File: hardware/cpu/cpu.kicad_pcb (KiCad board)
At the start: 4 copper layers, 172.7 x 106.7 mm, 64 parts, among them J1 Conn_02x20_Odd_Even, J2 Conn_01x06, J3 Conn_01x06, J4 Conn_02x05_Odd_Even, J5 Conn_01x02, J6 Conn_02x20_Odd_Even, SW1 SW_Push, U1 74AS74, U10 74LS157, U11 Z80-DART, U12 74HCT04, U13 74LS32, U14 CTC, U15 74HCT04, U16 uA7805, U17 74AS74, U18 74AS74, U2 74LS138, U3 Z80CPU, U4 AT28C256, U5 74LS670, U6 74HC14, U7 74LS670, U8 AS6C4008, U9 Z80-PIO, X1 7.3728MHz

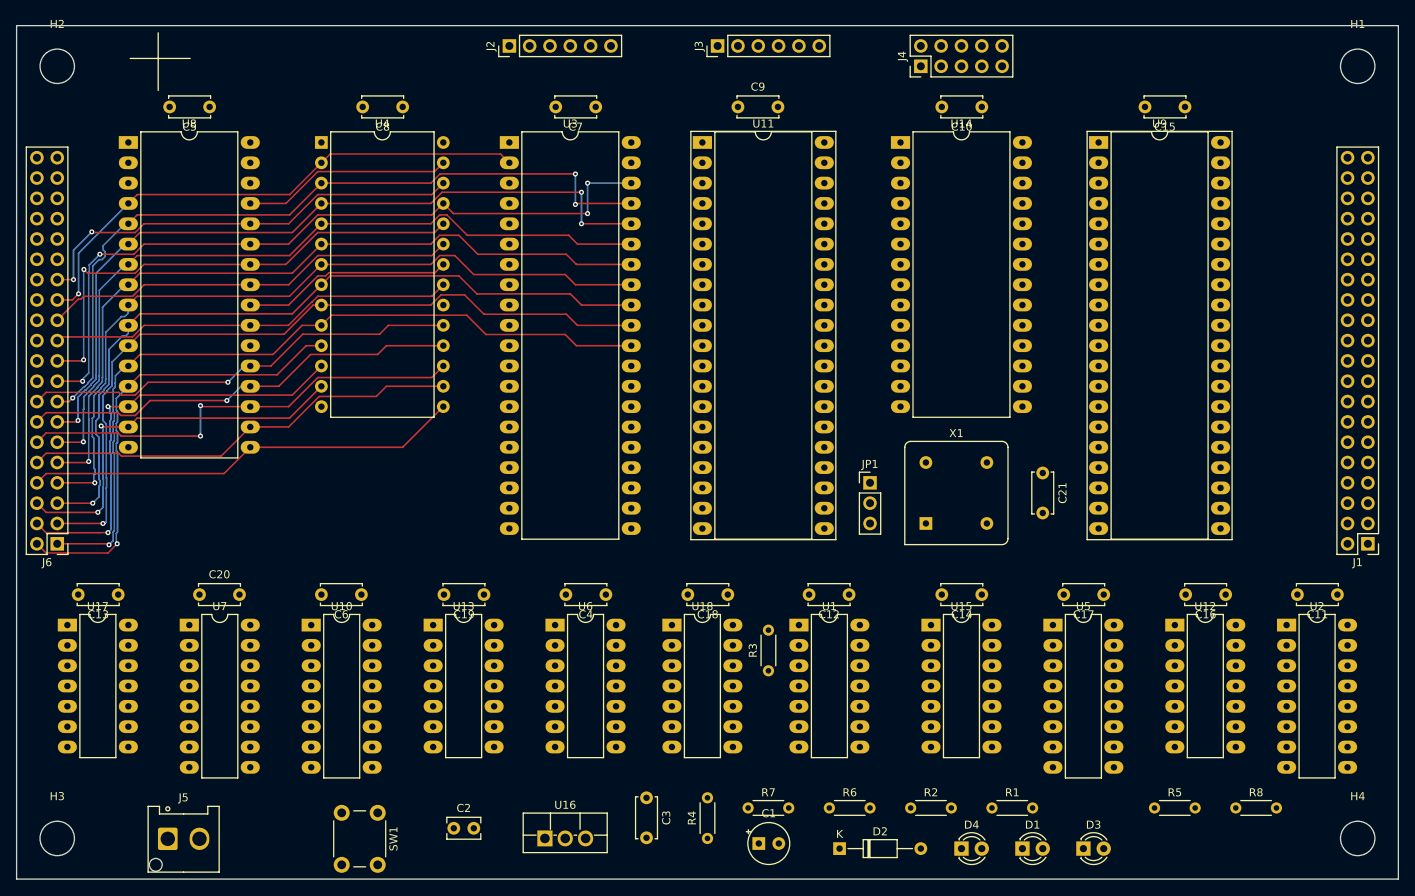
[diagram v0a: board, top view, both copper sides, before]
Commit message: updating
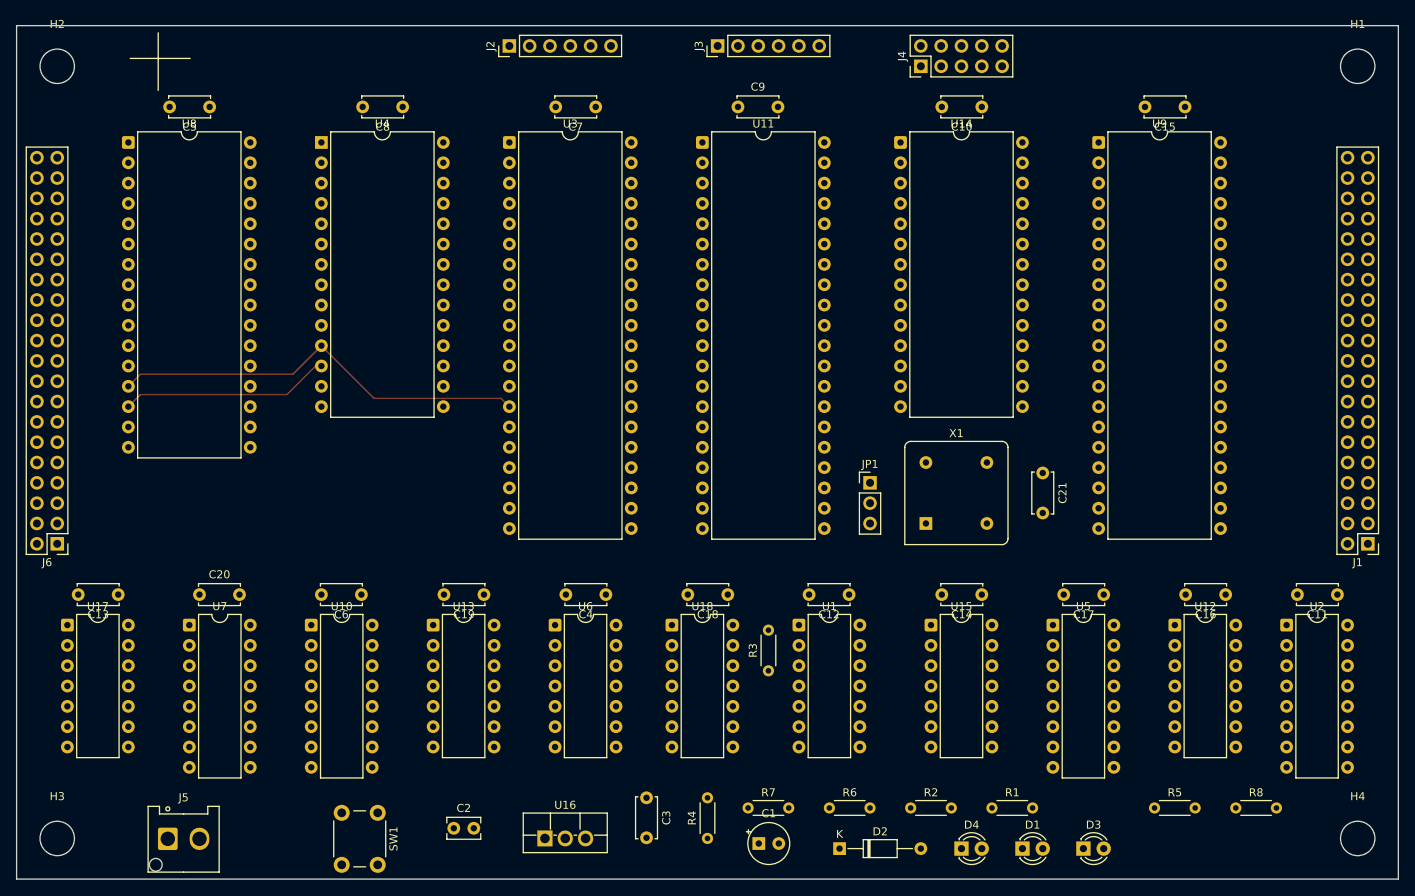
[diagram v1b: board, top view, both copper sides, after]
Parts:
- U1, U12, U13, U15, U17, U18, U6: footprint Package_DIP:DIP-14_W7.62mm_LongPads -> Package_DIP:DIP-14_W7.62mm
- U10, U2, U5, U7: footprint Package_DIP:DIP-16_W7.62mm_LongPads -> Package_DIP:DIP-16_W7.62mm
- U11, U9: footprint Package_DIP:DIP-40_W15.24mm_Socket_LongPads -> Package_DIP:DIP-40_W15.24mm
- U14: footprint Package_DIP:DIP-28_W15.24mm_LongPads -> Package_DIP:DIP-28_W15.24mm
- U3: footprint Package_DIP:DIP-40_W15.24mm_LongPads -> Package_DIP:DIP-40_W15.24mm
- U8: footprint Package_DIP:DIP-32_W15.24mm_LongPads -> Package_DIP:DIP-32_W15.24mm
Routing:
- net /A0: track 97.5 -> 0.00 mm, vias 1 -> 0
- net /A6: track 97.1 -> 0.00 mm, vias 3 -> 0
- net /A1: track 97.0 -> 0.00 mm, vias 1 -> 0
- net /A7: track 96.8 -> 0.00 mm, vias 3 -> 0
- net /A3: track 96.2 -> 0.00 mm, vias 1 -> 0
- net /A2: track 96.1 -> 0.00 mm, vias 1 -> 0
- net /A4: track 95.7 -> 0.00 mm, vias 1 -> 0
- net /A5: track 95.0 -> 0.00 mm, vias 1 -> 0
- net /A8: track 93.3 -> 0.00 mm, vias 4 -> 0
- net /A12: track 67.5 -> 0.00 mm, vias 1 -> 0
- net /A9: track 62.3 -> 0.00 mm, vias 2 -> 0
- net /D5: track 57.4 -> 0.00 mm, vias 2 -> 0
- net /A13: track 55.5 -> 0.00 mm, vias 2 -> 0
- net /D6: track 55.0 -> 0.00 mm, vias 1 -> 0
- net /D4: track 55.0 -> 0.00 mm
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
